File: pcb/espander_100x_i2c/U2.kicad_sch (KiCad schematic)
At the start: 4 parts, among them J5 DG127A-5.08-06P-14-00AH, J6 DG127A-5.08-06P-14-00AH, J7 DG127A-5.08-06P-14-00AH, U2 MCP23017_SP

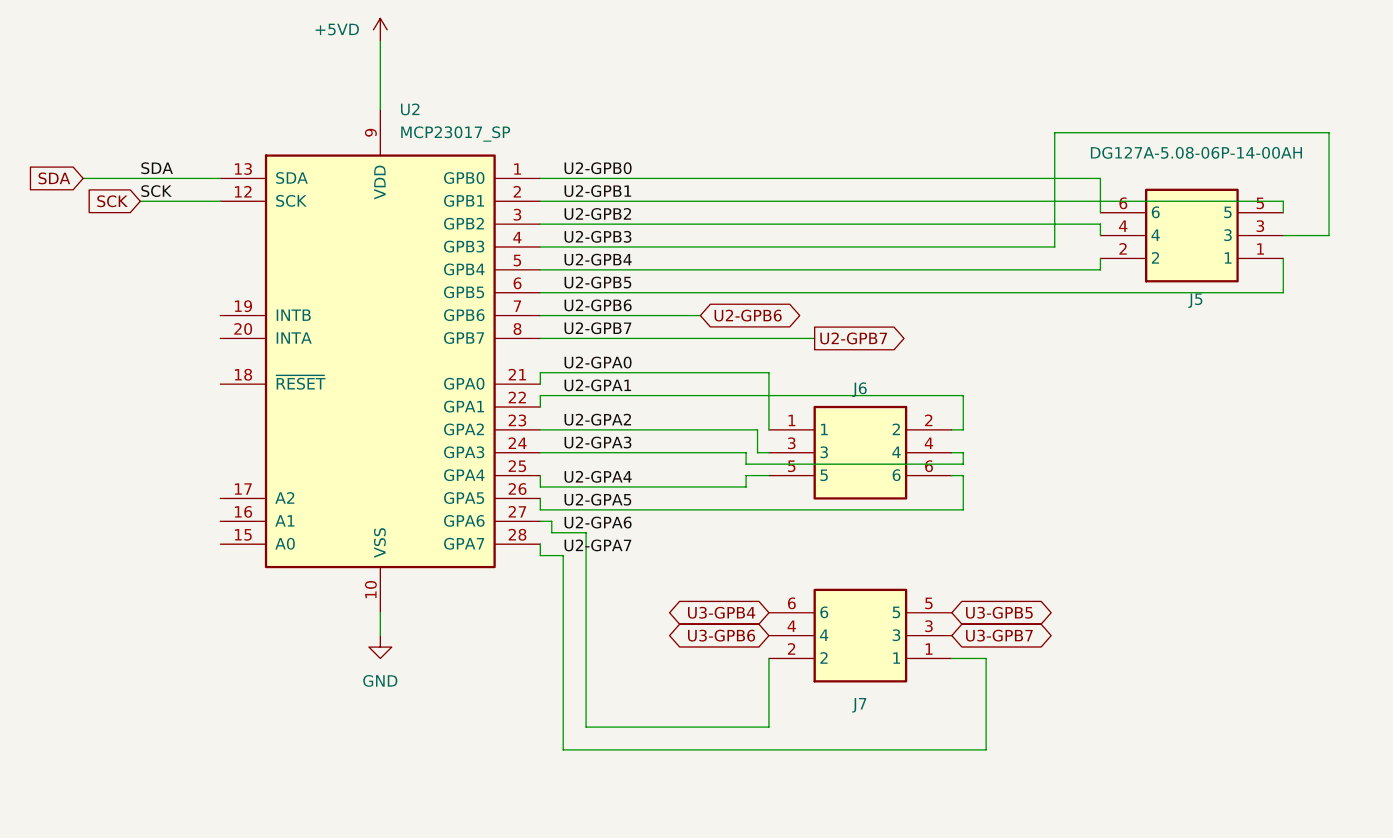
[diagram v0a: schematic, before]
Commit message: Refactor code structure for improved readability and maintainability
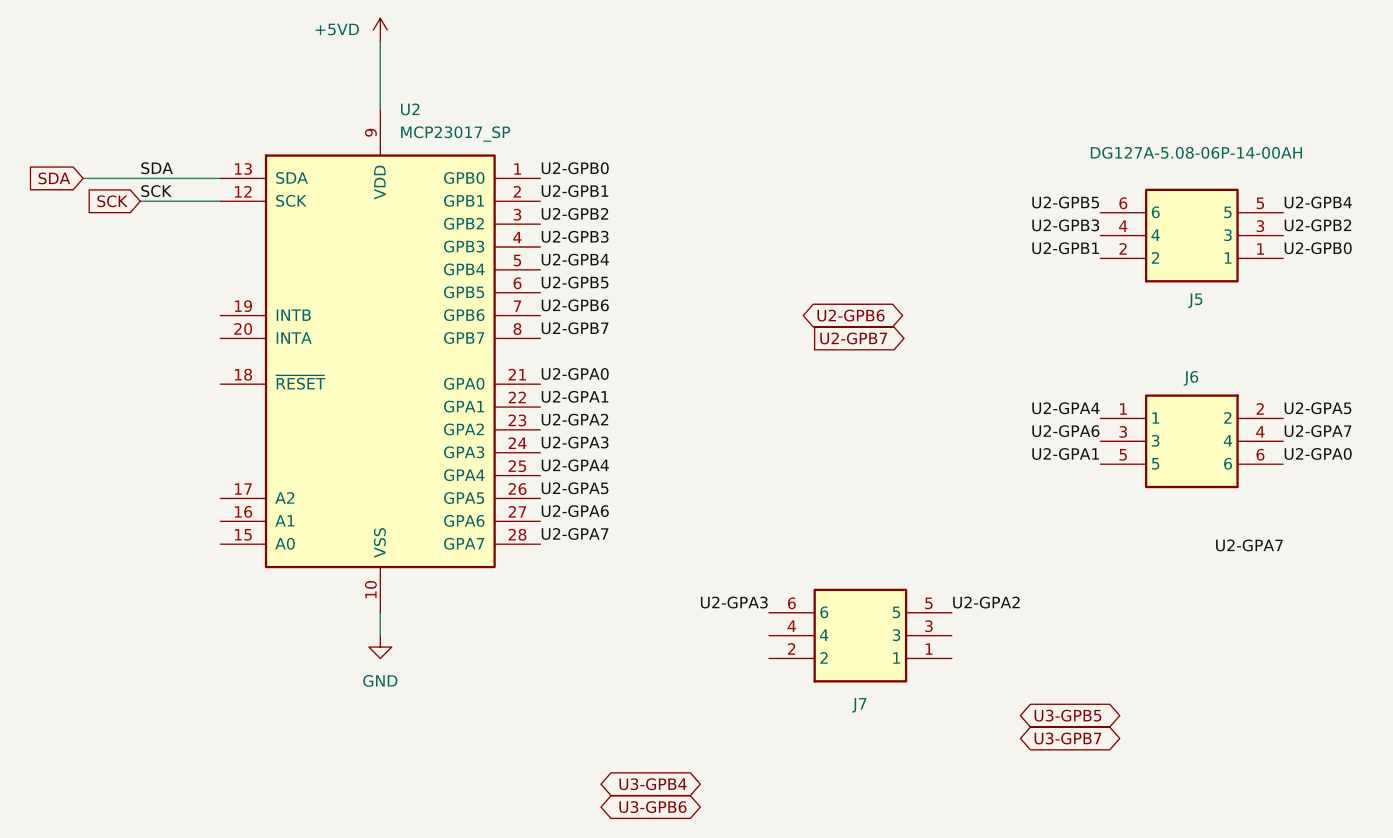
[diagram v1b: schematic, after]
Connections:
- net U2-GPA0: now also J6.6; no longer J6.1
- net U2-GPA1: now also J6.5; no longer J6.2
- net U2-GPA2: now also J7.5; no longer J6.3
- net U2-GPA3: now also J7.6; no longer J6.4
- net U2-GPA4: now also J6.1; no longer J6.5
- net U2-GPA5: now also J6.2; no longer J6.6
- net U2-GPA6: now also J6.3; no longer J7.2
- net U2-GPA7: now also J6.4; no longer J7.1
- net U2-GPB0: now also J5.1; no longer J5.6
- net U2-GPB1: now also J5.2; no longer J5.5
- net U2-GPB2: now also J5.3; no longer J5.4
- net U2-GPB3: now also J5.4; no longer J5.3
- net U2-GPB4: now also J5.5; no longer J5.2
- net U2-GPB5: now also J5.6; no longer J5.1
- net U3-GPB4: no longer J7.6
- net U3-GPB5: no longer J7.5
- net U3-GPB6: no longer J7.4
- net U3-GPB7: no longer J7.3
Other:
- moved on the sheet: J6

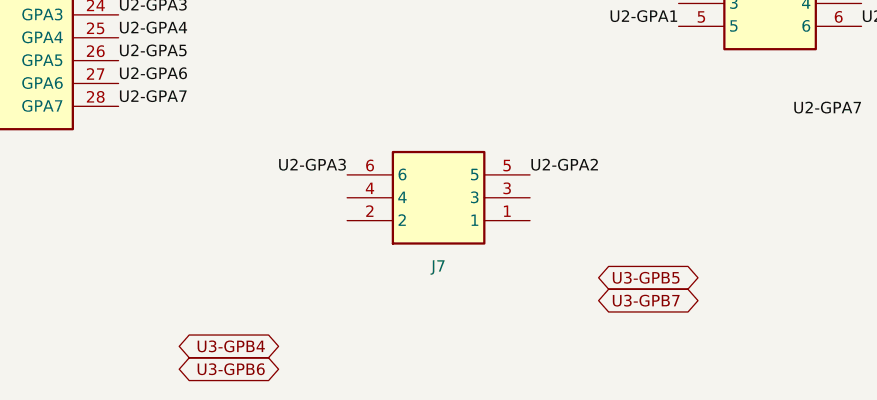
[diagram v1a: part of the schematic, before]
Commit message: RESYNC
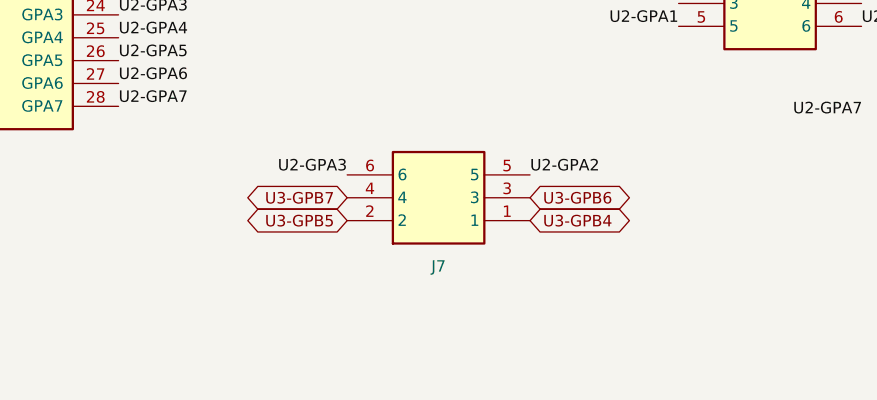
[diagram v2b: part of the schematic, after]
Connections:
- net U3-GPB4: now also J7.1
- net U3-GPB5: now also J7.2
- net U3-GPB6: now also J7.3
- net U3-GPB7: now also J7.4
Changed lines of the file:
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@@
 	(global_label "U3-GPB6"
 		(shape bidirectional)
-		(at 102.87 116.84 180)
+		(at 130.81 97.79 0)
 		(fields_autoplaced yes)
 		(effects
@@
 				(size 1.27 1.27)
 			)
-			(justify right)
+			(justify left)
 		)
 		(property "Intersheetrefs" "${INTERSHEET_REFS}"
-			(at 89.6416 116.84 0)
+			(at 144.0384 97.79 0)
 			(effects
 				(font
 					(size 1.27 1.27)
 				)
-				(justify right)
+				(justify left)
 				(hide yes)
 			)
@@
 	(global_label "U3-GPB4"
 		(shape bidirectional)
-		(at 102.87 114.3 180)
+		(at 130.81 100.33 0)
 		(fields_autoplaced yes)
 		(effects
@@
 				(size 1.27 1.27)
 			)
-			(justify right)
+			(justify left)
 		)
 		(property "Intersheetrefs" "${INTERSHEET_REFS}"
-			(at 89.6416 114.3 0)
+			(at 144.0384 100.33 0)
 			(effects
 				(font
 					(size 1.27 1.27)
 				)
-				(justify right)
+				(justify left)
 				(hide yes)
 			)
@@
 	(global_label "U3-GPB5"
 		(shape bidirectional)
-		(at 138.43 106.68 0)
+		(at 110.49 100.33 180)
 		(fields_autoplaced yes)
 		(effects
@@
 				(size 1.27 1.27)
 			)
-			(justify left)
+			(justify right)
 		)
 		(property "Intersheetrefs" "${INTERSHEET_REFS}"
-			(at 151.6584 106.68 0)
+			(at 97.2616 100.33 0)
 			(effects
 				(font
 					(size 1.27 1.27)
 				)
-				(justify left)
+				(justify right)
 				(hide yes)
 			)
@@
 	(global_label "U3-GPB7"
 		(shape bidirectional)
-		(at 138.43 109.22 0)
+		(at 110.49 97.79 180)
 		(fields_autoplaced yes)
 		(effects
@@
 				(size 1.27 1.27)
 			)
-			(justify left)
+			(justify right)
 		)
 		(property "Intersheetrefs" "${INTERSHEET_REFS}"
-			(at 151.6584 109.22 0)
+			(at 97.2616 97.79 0)
 			(effects
 				(font
 					(size 1.27 1.27)
 				)
-				(justify left)
+				(justify right)
 				(hide yes)
 			)

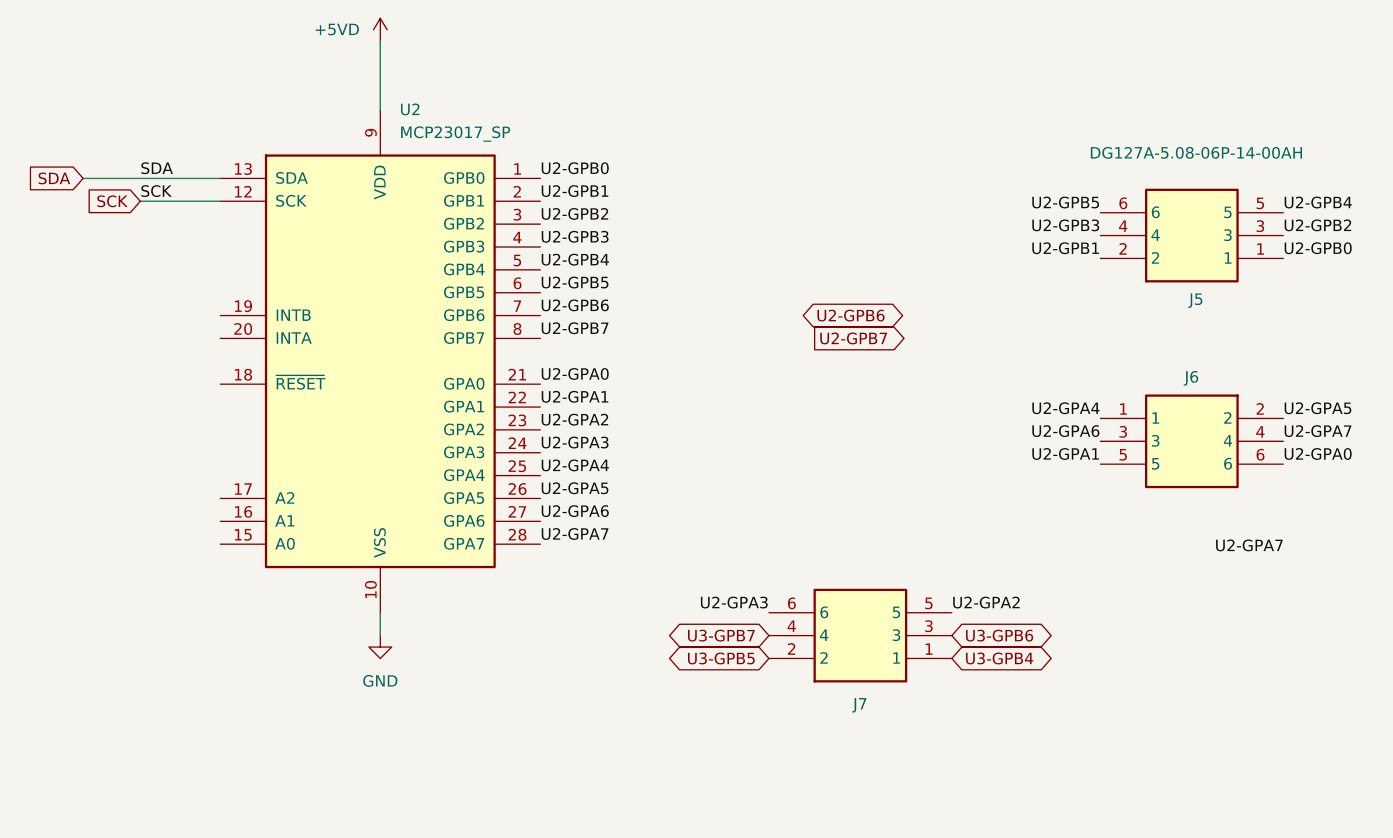
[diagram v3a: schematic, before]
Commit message: resync
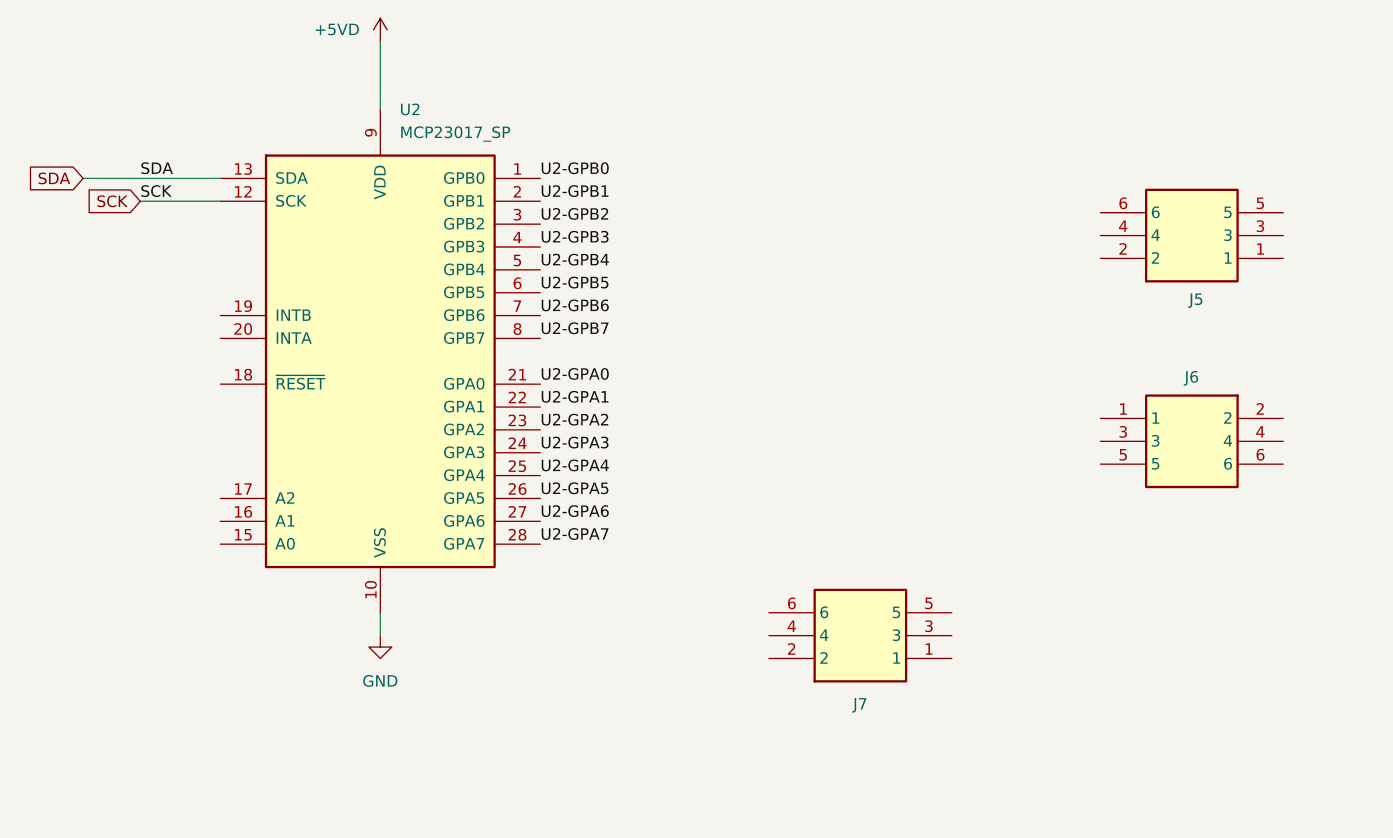
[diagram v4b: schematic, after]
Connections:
- net U2-GPA0: no longer J6.6
- net U2-GPA1: no longer J6.5
- net U2-GPA2: no longer J7.5
- net U2-GPA3: no longer J7.6
- net U2-GPA4: no longer J6.1
- net U2-GPA5: no longer J6.2
- net U2-GPA6: no longer J6.3
- net U2-GPA7: no longer J6.4
- net U2-GPB0: no longer J5.1
- net U2-GPB1: no longer J5.2
- net U2-GPB2: no longer J5.3
- net U2-GPB3: no longer J5.4
- net U2-GPB4: no longer J5.5
- net U2-GPB5: no longer J5.6
- net U3-GPB4: no longer names the net of J7.1
- net U3-GPB5: no longer names the net of J7.2
- net U3-GPB6: no longer names the net of J7.3
- net U3-GPB7: no longer names the net of J7.4
